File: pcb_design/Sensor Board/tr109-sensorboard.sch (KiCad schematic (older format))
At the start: 52 parts, among them J1 Conn_01x01_Female, J2 Conn_01x01_Female, J47 Raspberry_Pi_2_3, U1 BME680, U2 74HC595, U3 AMG8833, U4 LIS3MDLTR

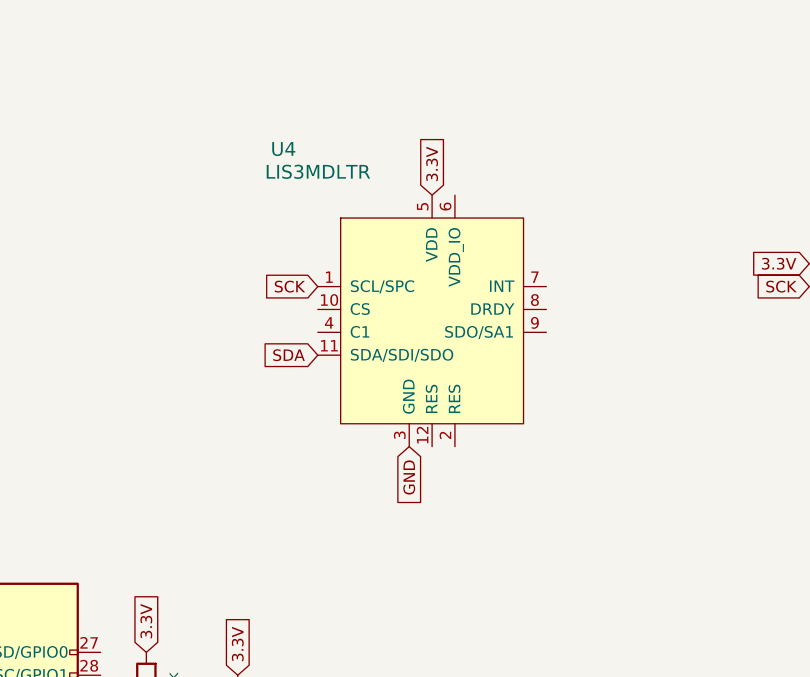
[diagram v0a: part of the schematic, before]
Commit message: sensor board revisions
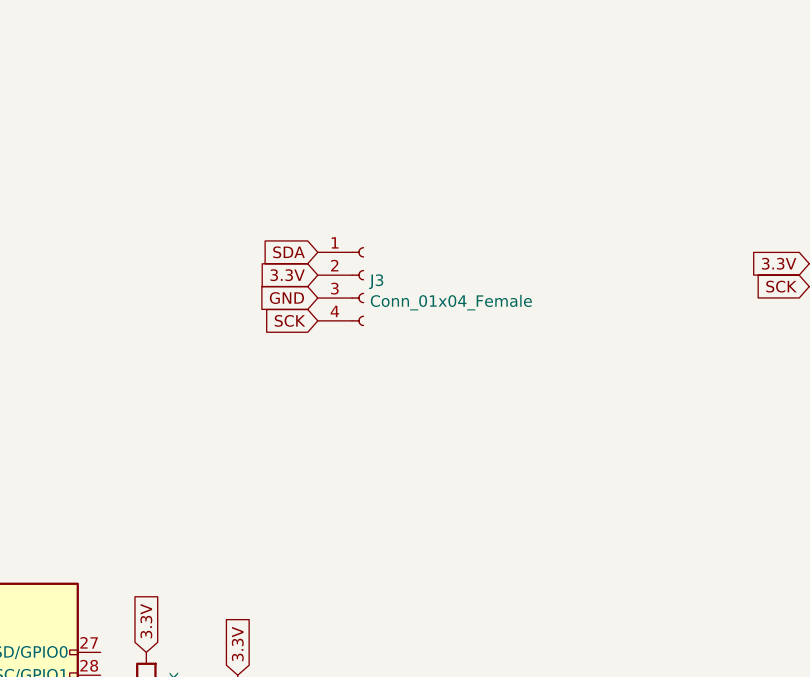
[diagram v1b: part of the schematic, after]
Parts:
- removed U4: LIS3MDLTR, digikey-footprints:VFLGA-12_2x2mm, symbol dk_Magnetic-Sensors-Linear-Compass-ICs:LIS3MDLTR
- added J3: Conn_01x04_Female, Connector_PinHeader_1.00mm:PinHeader_1x04_P1.00mm_Vertical, symbol Connector:Conn_01x04_Female
- J1, J2: footprint Connector_Wire:SolderWirePad_1x01_SMD_1x2mm -> TestPoint:TestPoint_Pad_1.0x1.0mm
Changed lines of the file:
@@
 Text GLabel 5850 1500 0    50   Input ~ 0
 3.3V
-Text GLabel 3700 1900 0    50   Input ~ 0
-SDA
-Text GLabel 3700 1600 0    50   Input ~ 0
-SCK
-Text GLabel 4100 2300 3    50   Input ~ 0
-GND
-Text GLabel 4200 1200 1    50   Input ~ 0
-3.3V
-$Comp
-L dk_Magnetic-Sensors-Linear-Compass-ICs:LIS3MDLTR U4
-U 1 1 5F5C68D1
-P 4200 1700
-F 0 "U4" H 3550 2400 60  0000 C CNN
-F 1 "LIS3MDLTR" H 3700 2300 60  0000 C CNN
-F 2 "digikey-footprints:VFLGA-12_2x2mm" H 4400 1900 60  0001 L CNN
-F 3 "http://www.st.com/content/ccc/resource/technical/document/datasheet/54/2a/85/76/e3/97/42/18/DM00075867.pdf/files/DM00075867.pdf/jcr:content/translations/en.DM00075867.pdf" H 4400 2000 60  0001 L CNN
-F 4 "497-13892-1-ND" H 4400 2100 60  0001 L CNN "Digi-Key_PN"
-F 5 "LIS3MDLTR" H 4400 2200 60  0001 L CNN "MPN"
-F 6 "Sensors, Transducers" H 4400 2300 60  0001 L CNN "Category"
-F 7 "Magnetic Sensors - Linear, Compass (ICs)" H 4400 2400 60  0001 L CNN "Family"
-F 8 "http://www.st.com/content/ccc/resource/technical/document/datasheet/54/2a/85/76/e3/97/42/18/DM00075867.pdf/files/DM00075867.pdf/jcr:content/translations/en.DM00075867.pdf" H 4400 2500 60  0001 L CNN "DK_Datasheet_Link"
-F 9 "/product-detail/en/stmicroelectronics/LIS3MDLTR/497-13892-1-ND/4309737" H 4400 2600 60  0001 L CNN "DK_Detail_Page"
-F 10 "SENSOR MR I2C/SPI 12LGA" H 4400 2700 60  0001 L CNN "Description"
-F 11 "STMicroelectronics" H 4400 2800 60  0001 L CNN "Manufacturer"
-F 12 "Active" H 4400 2900 60  0001 L CNN "Status"
-	1    4200 1700
-	1    0    0    -1
-$EndComp
 Text GLabel 4550 6400 2    50   Input ~ 0
 GND
@@
 F 0 "J2" H 5728 5626 50  0000 L CNN
 F 1 "Conn_01x01_Female" H 5728 5535 50  0000 L CNN
-F 2 "Connector_Wire:SolderWirePad_1x01_SMD_1x2mm" H 5700 5600 50  0001 C CNN
+F 2 "TestPoint:TestPoint_Pad_1.0x1.0mm" H 5700 5600 50  0001 C CNN
 F 3 "~" H 5700 5600 50  0001 C CNN
 	1    5700 5600
@@
 F 0 "J1" H 5728 5276 50  0000 L CNN
 F 1 "Conn_01x01_Female" H 5728 5185 50  0000 L CNN
-F 2 "Connector_Wire:SolderWirePad_1x01_SMD_1x2mm" H 5700 5250 50  0001 C CNN
+F 2 "TestPoint:TestPoint_Pad_1.0x1.0mm" H 5700 5250 50  0001 C CNN
 F 3 "~" H 5700 5250 50  0001 C CNN
 	1    5700 5250
@@
 Text GLabel 6750 1600 2    50   Input ~ 0
 GND
+$Comp
+L Connector:Conn_01x04_Female J3
+U 1 1 60B3C235
+P 3900 1550
+F 0 "J3" H 3928 1526 50  0000 L CNN
+F 1 "Conn_01x04_Female" H 3928 1435 50  0000 L CNN
+F 2 "Connector_PinHeader_1.00mm:PinHeader_1x04_P1.00mm_Vertical" H 3900 1550 50  0001 C CNN
+F 3 "~" H 3900 1550 50  0001 C CNN
+	1    3900 1550
+	1    0    0    -1
+$EndComp
+Text GLabel 3700 1450 0    50   Input ~ 0
+SDA
+Text GLabel 3700 1750 0    50   Input ~ 0
+SCK
+Text GLabel 3700 1550 0    50   Input ~ 0
+3.3V
+Text GLabel 3700 1650 0    50   Input ~ 0
+GND
 $EndSCHEMATC
